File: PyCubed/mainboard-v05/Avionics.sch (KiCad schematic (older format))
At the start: 33 parts, among them SW1 KMR231NG LFS, U1 MAX706RESA, U2 ATSAMD51J19A-AU, U3 BMX160, Y1 32.768kHz

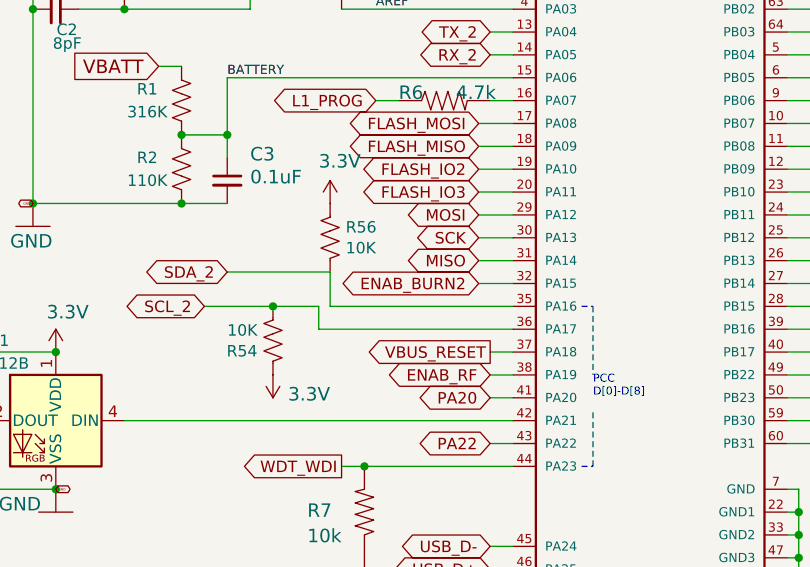
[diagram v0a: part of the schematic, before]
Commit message: pycubed finished, awaiting review
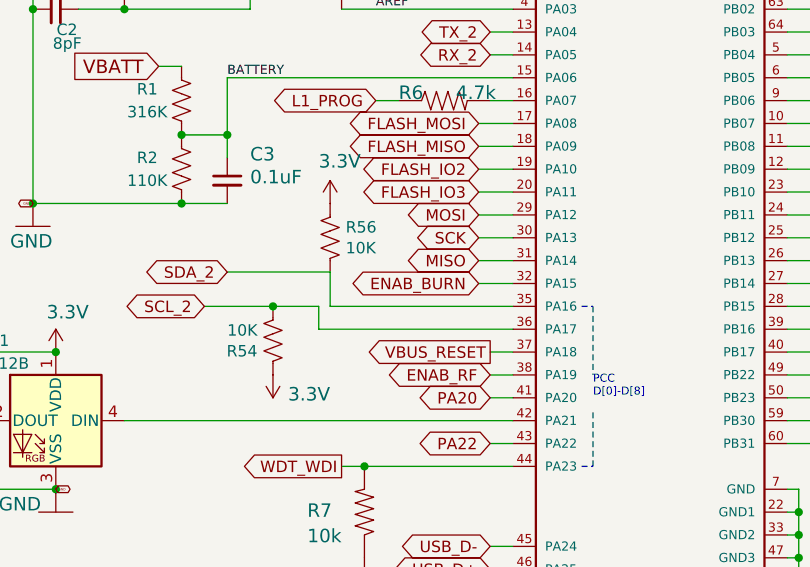
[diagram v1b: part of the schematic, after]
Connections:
- net ENAB_BURN2 renamed ENAB_BURN
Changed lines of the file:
@@
 ENAB_GPS
 Text GLabel 3500 5650 0    50   BiDi ~ 0
-ENAB_BURN2
+ENAB_BURN
 Text GLabel 5000 6350 2    50   BiDi ~ 0
 PB31
